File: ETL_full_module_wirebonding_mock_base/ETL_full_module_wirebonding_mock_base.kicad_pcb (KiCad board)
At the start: 2 copper layers, 56.5 x 43.1 mm, 12 parts

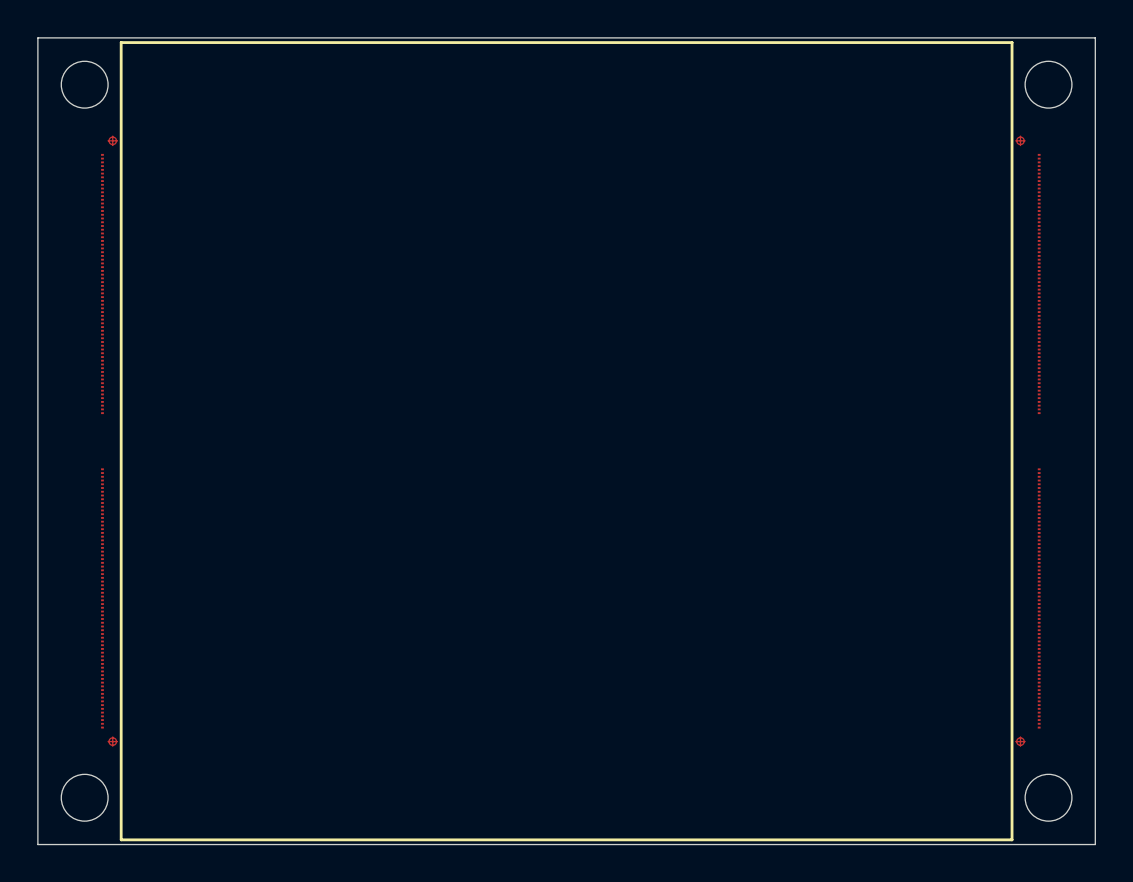
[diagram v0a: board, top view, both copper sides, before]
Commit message: Updates ETL_full_module_wirebonding_mock_base and top
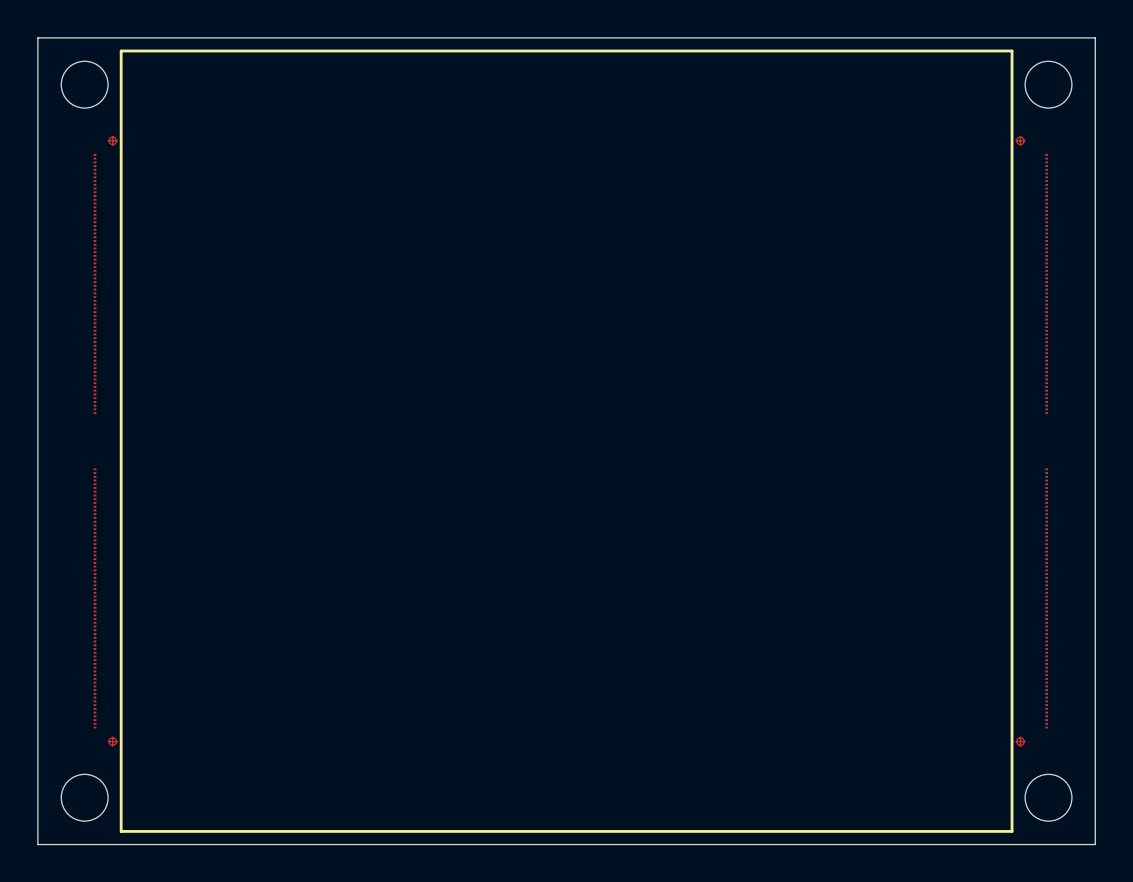
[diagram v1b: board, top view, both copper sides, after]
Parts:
- moved ETROC** 0.40 mm to (3.05, 6.25)
- moved ETROC** 0.40 mm to (3.05, 36.9)
- moved ETROC** 0.40 mm to (53.9, 36.9)
- moved ETROC** 0.40 mm to (53.9, 6.25)
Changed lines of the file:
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@@
   (general
     (thickness 1.6)
-    (drawings 12)
+    (drawings 13)
     (tracks 0)
     (zones 0)
@@
     (pad_to_mask_clearance 0.05)
     (aux_axis_origin 0 0)
-    (visible_elements FFFFFF7F)
+    (visible_elements 7FFFFFFF)
     (pcbplotparams
-      (layerselection 0x010fc_ffffffff)
+      (layerselection 0x010a8_7fffffff)
       (usegerberextensions false)
       (usegerberattributes true)
@@
       (outputformat 1)
       (mirror false)
-      (drillshape 1)
+      (drillshape 0)
       (scaleselection 1)
-      (outputdirectory ""))
+      (outputdirectory "fab_outputs/"))
   )
   (net 0 "")
@@
       (effects (font (size 1 1) (thickness 0.15)))
     )
+    (fp_circle (center 0 0) (end 0.01 0) (layer F.Mask) (width 0.6))
+    (fp_line (start 0.25 0) (end -0.25 0) (layer F.Cu) (width 0.07))
+    (fp_line (start 0 -0.25) (end 0 0.25) (layer F.Cu) (width 0.07))
     (fp_circle (center 0 0) (end 0.2 0) (layer F.Cu) (width 0.07))
-    (fp_line (start 0 -0.25) (end 0 0.25) (layer F.Cu) (width 0.07))
-    (fp_line (start 0.25 0) (end -0.25 0) (layer F.Cu) (width 0.07))
-    (fp_circle (center 0 0) (end 0.01 0) (layer F.Mask) (width 0.6))
   )
   (module unl_silab:crossed_circle_fiducial (layer F.Cu)
@@
       (effects (font (size 1 1) (thickness 0.15)))
     )
+    (fp_circle (center 0 0) (end 0.01 0) (layer F.Mask) (width 0.6))
+    (fp_line (start 0.25 0) (end -0.25 0) (layer F.Cu) (width 0.07))
+    (fp_line (start 0 -0.25) (end 0 0.25) (layer F.Cu) (width 0.07))
     (fp_circle (center 0 0) (end 0.2 0) (layer F.Cu) (width 0.07))
-    (fp_line (start 0 -0.25) (end 0 0.25) (layer F.Cu) (width 0.07))
-    (fp_line (start 0.25 0) (end -0.25 0) (layer F.Cu) (width 0.07))
-    (fp_circle (center 0 0) (end 0.01 0) (layer F.Mask) (width 0.6))
   )
   (module unl_silab:crossed_circle_fiducial (layer F.Cu)
@@
       (effects (font (size 1 1) (thickness 0.15)))
     )
+    (fp_circle (center 0 0) (end 0.01 0) (layer F.Mask) (width 0.6))
+    (fp_line (start 0.25 0) (end -0.25 0) (layer F.Cu) (width 0.07))
+    (fp_line (start 0 -0.25) (end 0 0.25) (layer F.Cu) (width 0.07))
     (fp_circle (center 0 0) (end 0.2 0) (layer F.Cu) (width 0.07))
-    (fp_line (start 0 -0.25) (end 0 0.25) (layer F.Cu) (width 0.07))
-    (fp_line (start 0.25 0) (end -0.25 0) (layer F.Cu) (width 0.07))
-    (fp_circle (center 0 0) (end 0.01 0) (layer F.Mask) (width 0.6))
   )
   (module MountingHole:MountingHole_2.5mm (layer F.Cu)
@@
       (effects (font (size 1 1) (thickness 0.15)))
     )
+    (fp_circle (center 0 0) (end 2.75 0) (layer F.CrtYd) (width 0.05))
     (fp_circle (center 0 0) (end 2.5 0) (layer Cmts.User) (width 0.15))
-    (fp_circle (center 0 0) (end 2.75 0) (layer F.CrtYd) (width 0.05))
     (fp_text user %R (at 0.3 0) (layer F.Fab)
       (effects (font (size 1 1) (thickness 0.15)))
@@
       (effects (font (size 1 1) (thickness 0.15)))
     )
+    (fp_circle (center 0 0) (end 2.75 0) (layer F.CrtYd) (width 0.05))
     (fp_circle (center 0 0) (end 2.5 0) (layer Cmts.User) (width 0.15))
-    (fp_circle (center 0 0) (end 2.75 0) (layer F.CrtYd) (width 0.05))
     (fp_text user %R (at 0.3 0) (layer F.Fab)
       (effects (font (size 1 1) (thickness 0.15)))
@@
       (effects (font (size 1 1) (thickness 0.15)))
     )
+    (fp_circle (center 0 0) (end 2.75 0) (layer F.CrtYd) (width 0.05))
     (fp_circle (center 0 0) (end 2.5 0) (layer Cmts.User) (width 0.15))
-    (fp_circle (center 0 0) (end 2.75 0) (layer F.CrtYd) (width 0.05))
     (fp_text user %R (at 0.3 0) (layer F.Fab)
       (effects (font (size 1 1) (thickness 0.15)))
@@
       (effects (font (size 1 1) (thickness 0.15)))
     )
+    (fp_circle (center 0 0) (end 2.75 0) (layer F.CrtYd) (width 0.05))
+    (fp_circle (center 0 0) (end 2.5 0) (layer Cmts.User) (width 0.15))
     (fp_text user %R (at 0.3 0) (layer F.Fab)
       (effects (font (size 1 1) (thickness 0.15)))
     )
-    (fp_circle (center 0 0) (end 2.5 0) (layer Cmts.User) (width 0.15))
-    (fp_circle (center 0 0) (end 2.75 0) (layer F.CrtYd) (width 0.05))
     (pad 1 np_thru_hole circle (at 0 0) (size 2.5 2.5) (drill 2.5) (layers *.Cu *.Mask))
   )
@@
       (effects (font (size 1 1) (thickness 0.15)))
     )
+    (fp_circle (center 0 0) (end 0.01 0) (layer F.Mask) (width 0.6))
+    (fp_line (start 0.25 0) (end -0.25 0) (layer F.Cu) (width 0.07))
+    (fp_line (start 0 -0.25) (end 0 0.25) (layer F.Cu) (width 0.07))
     (fp_circle (center 0 0) (end 0.2 0) (layer F.Cu) (width 0.07))
-    (fp_line (start 0 -0.25) (end 0 0.25) (layer F.Cu) (width 0.07))
-    (fp_line (start 0.25 0) (end -0.25 0) (layer F.Cu) (width 0.07))
-    (fp_circle (center 0 0) (end 0.01 0) (layer F.Mask) (width 0.6))
   )
   (module unl_silab:ETROC_70pad_100x150um_200um_pitch (layer F.Cu)
-    (at 53.5 36.85 90)
+    (at 53.9 36.85 90)
     (fp_text reference ETROC** (at 0 0.5 90) (layer F.SilkS) hide
       (effects (font (size 1 1) (thickness 0.15)))
@@
   )
   (module unl_silab:ETROC_70pad_100x150um_200um_pitch (layer F.Cu)
-    (at 53.5 6.25 270)
+    (at 53.9 6.25 270)
     (fp_text reference ETROC** (at 0 0.5 90) (layer F.SilkS) hide
       (effects (font (size 1 1) (thickness 0.15)))
@@
   )
   (module unl_silab:ETROC_70pad_100x150um_200um_pitch (layer F.Cu)
-    (at 3.45 6.25 270)
+    (at 3.05 6.25 270)
     (fp_text reference ETROC** (at 0 0.5 90) (layer F.SilkS) hide
       (effects (font (size 1 1) (thickness 0.15)))
@@
   )
   (module unl_silab:ETROC_70pad_100x150um_200um_pitch (layer F.Cu)
-    (at 3.45 36.85 90)
+    (at 3.05 36.85 90)
     (fp_text reference ETROC** (at 0 0.5 90) (layer F.SilkS) hide
       (effects (font (size 1 1) (thickness 0.15)))
@@
     (pad 1 smd rect (at 0 0 90) (size 0.1 0.15) (layers F.Cu F.Mask))
   )
-  (dimension 40.850001 (width 0.15) (layer Dwgs.User)
-    (gr_text "40.850 mm" (at 48.95 22.424999 90) (layer Dwgs.User)
-      (effects (font (size 1 1) (thickness 0.15)))
-    )
-    (feature1 (pts (xy 52.05 1.999999) (xy 49.663579 1.999999)))
-    (feature2 (pts (xy 52.05 42.85) (xy 49.663579 42.85)))
-    (crossbar (pts (xy 50.25 42.85) (xy 50.25 1.999999)))
-    (arrow1a (pts (xy 50.25 1.999999) (xy 50.836421 3.126503)))
-    (arrow1b (pts (xy 50.25 1.999999) (xy 49.663579 3.126503)))
-    (arrow2a (pts (xy 50.25 42.85) (xy 50.836421 41.723496)))
-    (arrow2b (pts (xy 50.25 42.85) (xy 49.663579 41.723496)))
-  )
   (dimension 47.6 (width 0.15) (layer Dwgs.User)
-    (gr_text "47.600 mm" (at 28.25 3.299999) (layer Dwgs.User)
-      (effects (font (size 1 1) (thickness 0.15)))
-    )
-    (feature1 (pts (xy 52.05 0.25) (xy 52.05 2.58642)))
-    (feature2 (pts (xy 4.45 0.25) (xy 4.45 2.58642)))
-    (crossbar (pts (xy 4.45 1.999999) (xy 52.05 1.999999)))
-    (arrow1a (pts (xy 52.05 1.999999) (xy 50.923496 2.58642)))
-    (arrow1b (pts (xy 52.05 1.999999) (xy 50.923496 1.413578)))
-    (arrow2a (pts (xy 4.45 1.999999) (xy 5.576504 2.58642)))
-    (arrow2b (pts (xy 4.45 1.999999) (xy 5.576504 1.413578)))
+    (gr_text "47.600 mm" (at 28.25 2.95) (layer Dwgs.User)
+      (effects (font (size 1 1) (thickness 0.15)))
+    )
+    (feature1 (pts (xy 4.45 0.7) (xy 4.45 2.236421)))
+    (feature2 (pts (xy 52.05 0.7) (xy 52.05 2.236421)))
+    (crossbar (pts (xy 52.05 1.65) (xy 4.45 1.65)))
+    (arrow1a (pts (xy 4.45 1.65) (xy 5.576504 1.063579)))
+    (arrow1b (pts (xy 4.45 1.65) (xy 5.576504 2.236421)))
+    (arrow2a (pts (xy 52.05 1.65) (xy 50.923496 1.063579)))
+    (arrow2b (pts (xy 52.05 1.65) (xy 50.923496 2.236421)))
+  )
+  (dimension 41.7 (width 0.15) (layer Dwgs.User)
+    (gr_text "41.700 mm" (at 48.3 21.55 90) (layer Dwgs.User)
+      (effects (font (size 1 1) (thickness 0.15)))
+    )
+    (feature1 (pts (xy 52.05 0.7) (xy 49.013579 0.7)))
+    (feature2 (pts (xy 52.05 42.4) (xy 49.013579 42.4)))
+    (crossbar (pts (xy 49.6 42.4) (xy 49.6 0.7)))
+    (arrow1a (pts (xy 49.6 0.7) (xy 50.186421 1.826504)))
+    (arrow1b (pts (xy 49.6 0.7) (xy 49.013579 1.826504)))
+    (arrow2a (pts (xy 49.6 42.4) (xy 50.186421 41.273496)))
+    (arrow2b (pts (xy 49.6 42.4) (xy 49.013579 41.273496)))
+  )
+  (dimension 1.85 (width 0.15) (layer Dwgs.User)
+    (gr_text "1.850 mm" (at 52.975 -6.7) (layer Dwgs.User)
+      (effects (font (size 1 1) (thickness 0.15)))
+    )
+    (feature1 (pts (xy 52.05 6.25) (xy 52.05 -5.986421)))
+    (feature2 (pts (xy 53.9 6.25) (xy 53.9 -5.986421)))
+    (crossbar (pts (xy 53.9 -5.4) (xy 52.05 -5.4)))
+    (arrow1a (pts (xy 52.05 -5.4) (xy 53.176504 -5.986421)))
+    (arrow1b (pts (xy 52.05 -5.4) (xy 53.176504 -4.813579)))
+    (arrow2a (pts (xy 53.9 -5.4) (xy 52.773496 -5.986421)))
+    (arrow2b (pts (xy 53.9 -5.4) (xy 52.773496 -4.813579)))
   )
   (dimension 43.1 (width 0.15) (layer Dwgs.User)
@@
     (arrow2b (pts (xy 56.5 -1.749999) (xy 55.373496 -1.163578)))
   )
-  (gr_line (start 4.45 0.25) (end 52.05 0.25) (layer F.SilkS) (width 0.15))
-  (gr_line (start 52.05 0.25) (end 52.05 42.85) (layer F.SilkS) (width 0.15))
-  (gr_line (start 4.45 42.85) (end 52.05 42.85) (layer F.SilkS) (width 0.15))
-  (gr_line (start 4.45 0.25) (end 4.45 42.85) (layer F.SilkS) (width 0.15))
+  (gr_line (start 4.45 0.7) (end 52.05 0.7) (layer F.SilkS) (width 0.15))
+  (gr_line (start 52.05 0.7) (end 52.05 42.4) (layer F.SilkS) (width 0.15))
+  (gr_line (start 4.45 42.4) (end 52.05 42.4) (layer F.SilkS) (width 0.15))
+  (gr_line (start 4.45 0.7) (end 4.45 42.4) (layer F.SilkS) (width 0.15))
   (gr_line (start 0 0) (end 56.5 0) (layer Edge.Cuts) (width 0.05))
   (gr_line (start 56.5 0) (end 56.5 43.1) (layer Edge.Cuts) (width 0.05))
